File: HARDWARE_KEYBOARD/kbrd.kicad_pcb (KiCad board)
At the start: 2 copper layers, 65 x 46.5 mm, 24 parts, among them J1 USB_C_Receptacle_USB2.0_16P, J2 SWD, SW1 SW_SPST, SW2 SW_SPST, SW3 SW_SPST, SW4 SW_SPST, U1 STM32F103C8Tx, U2 AP2210N-3.3TRG1, Y1 Crystal_GND24

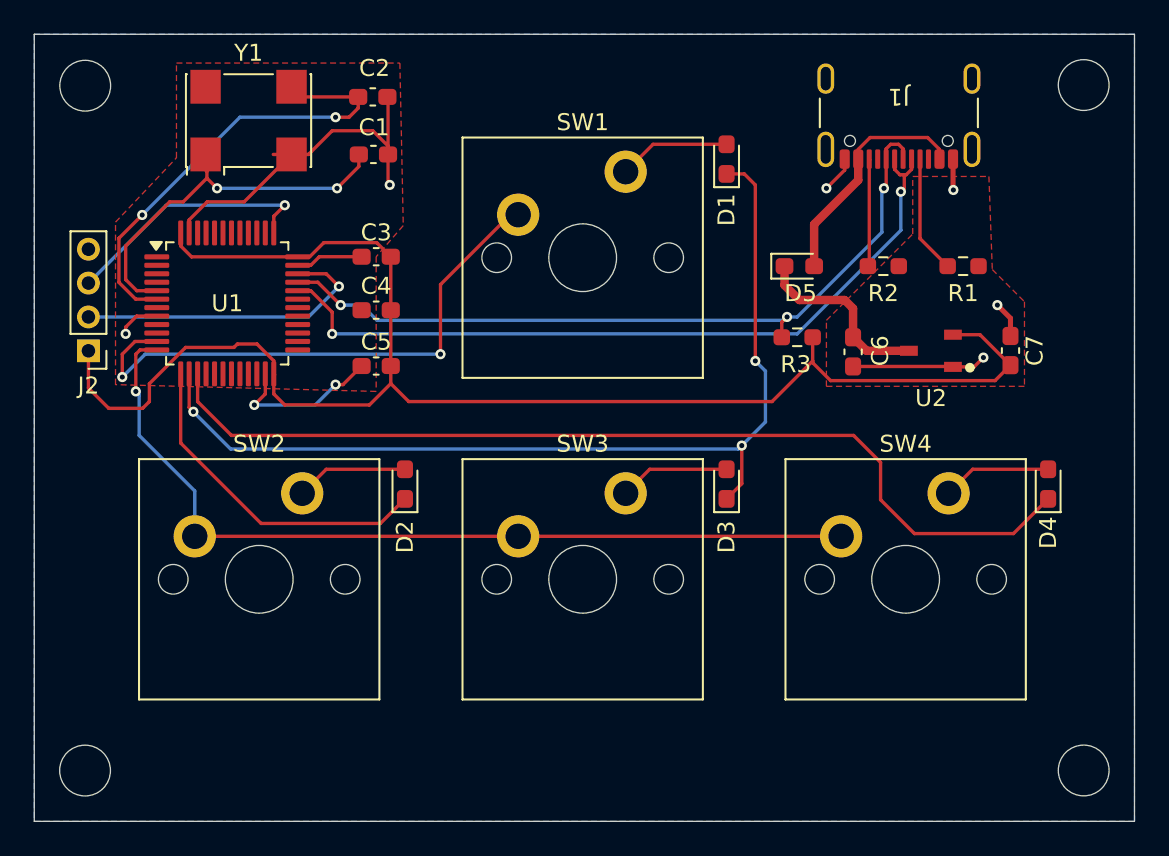
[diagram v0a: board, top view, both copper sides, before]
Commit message: Add gerber
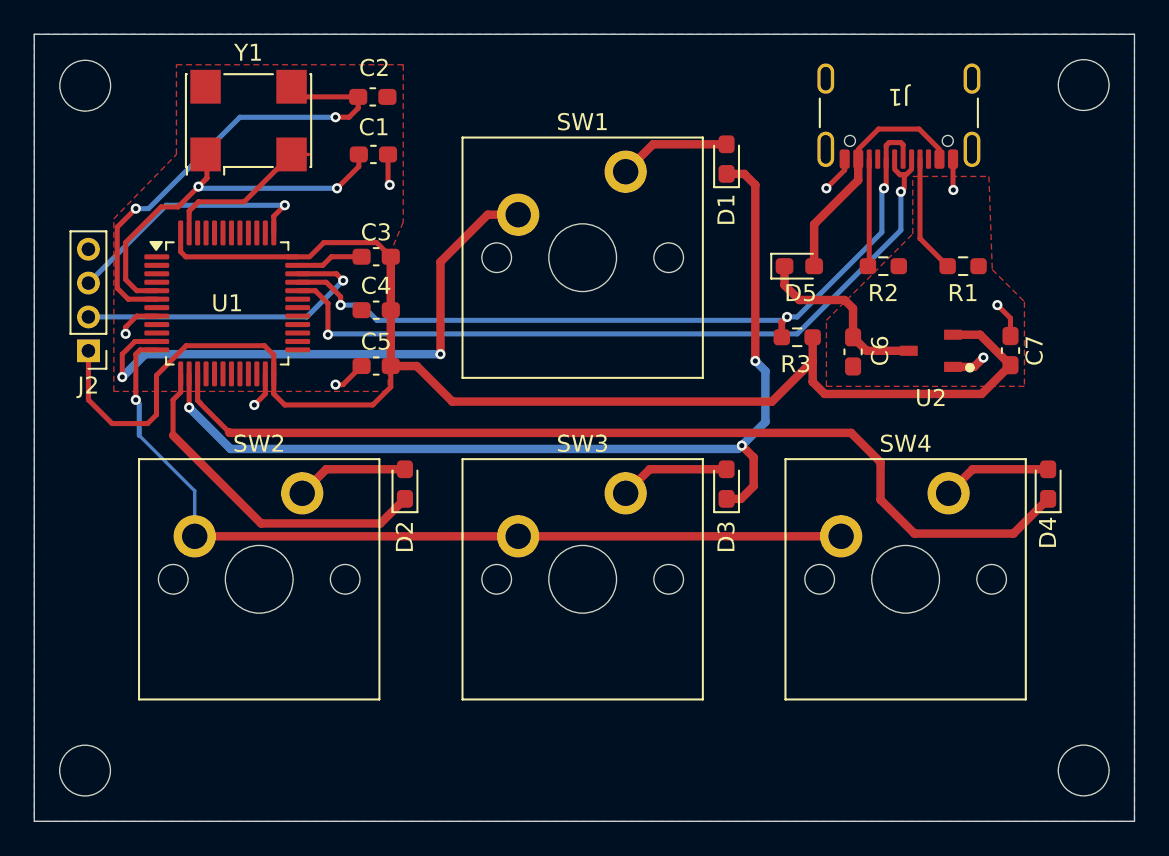
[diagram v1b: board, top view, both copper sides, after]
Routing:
- net GND: track 52.0 -> 30.6 mm
- net +3.3V: track 92.2 -> 95.6 mm
- net /OSC_IN: track 21.5 -> 22.7 mm
- net /COL2: track 57.5 -> 58.5 mm
- net /COL1: track 19.9 -> 20.7 mm
- net /ROW1: track 33.5 -> 34.3 mm
- net /OSC_OUT: track 27.4 -> 28.2 mm
- net /PA12: track 45.8 -> 46.4 mm
- net /SWDIO: track 18.3 -> 18.8 mm
